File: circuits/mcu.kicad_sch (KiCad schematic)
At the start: 35 parts, among them J1 USB_MINI_B, J2 USB_MINI_B, Q5 Q_L8050QLT1G, Q6 Q_L8550HQLT1G, SW1 SW_PUSH, SW2 SW_PUSH, SW3 SW_PUSH, U10 CP2102N-Axx-xQFN28, U9 ESP32-S3-WROOM-1

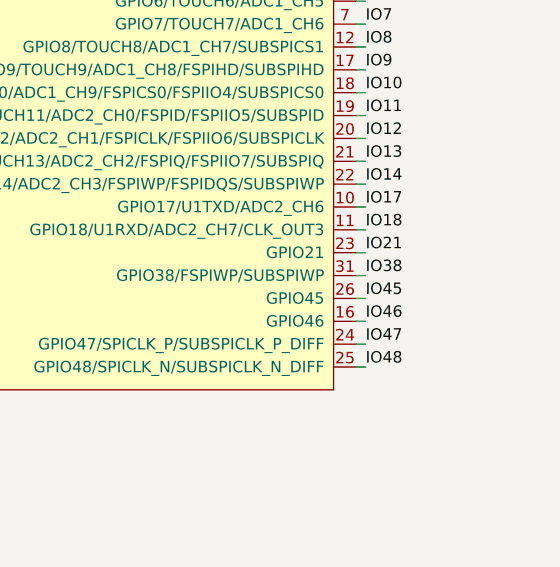
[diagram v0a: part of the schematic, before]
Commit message: save laser controller schematic and layout state
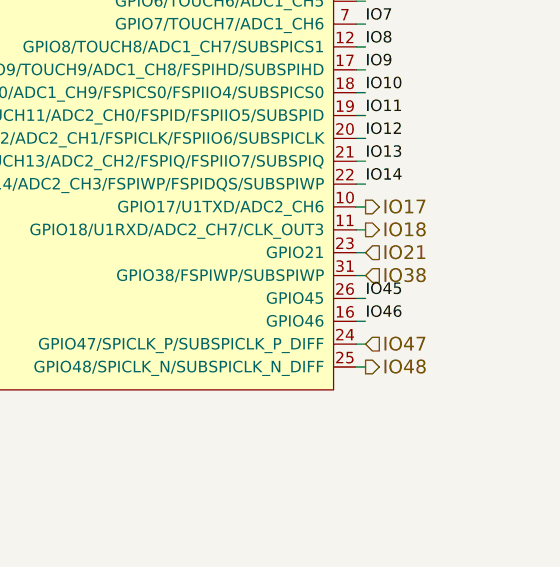
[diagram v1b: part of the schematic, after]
